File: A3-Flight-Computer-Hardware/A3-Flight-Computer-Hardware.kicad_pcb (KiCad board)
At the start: 2 copper layers, 50 x 50 mm, 57 parts, among them J1 BAT, J2 ST1W008S4ER1500, J3 USB_C_Receptacle_USB2.0_14P, J4 Cam 1, J5 Debug Header, J6 Cam 2, J7 Cam 3, J8 Telem, J9 CAN, SW1 BOOT, SW2 RST, U1 STM32H523RETx, U2 ADXL375BCCZ-RL7, U3 LSM6DSO32TR, U4 LPS22HBTR, U5 PTCAN3414DR, Y1 TSX-3225_16.0000MF18X-AC0, Y2 ECS-.327-9-34QCS-TR

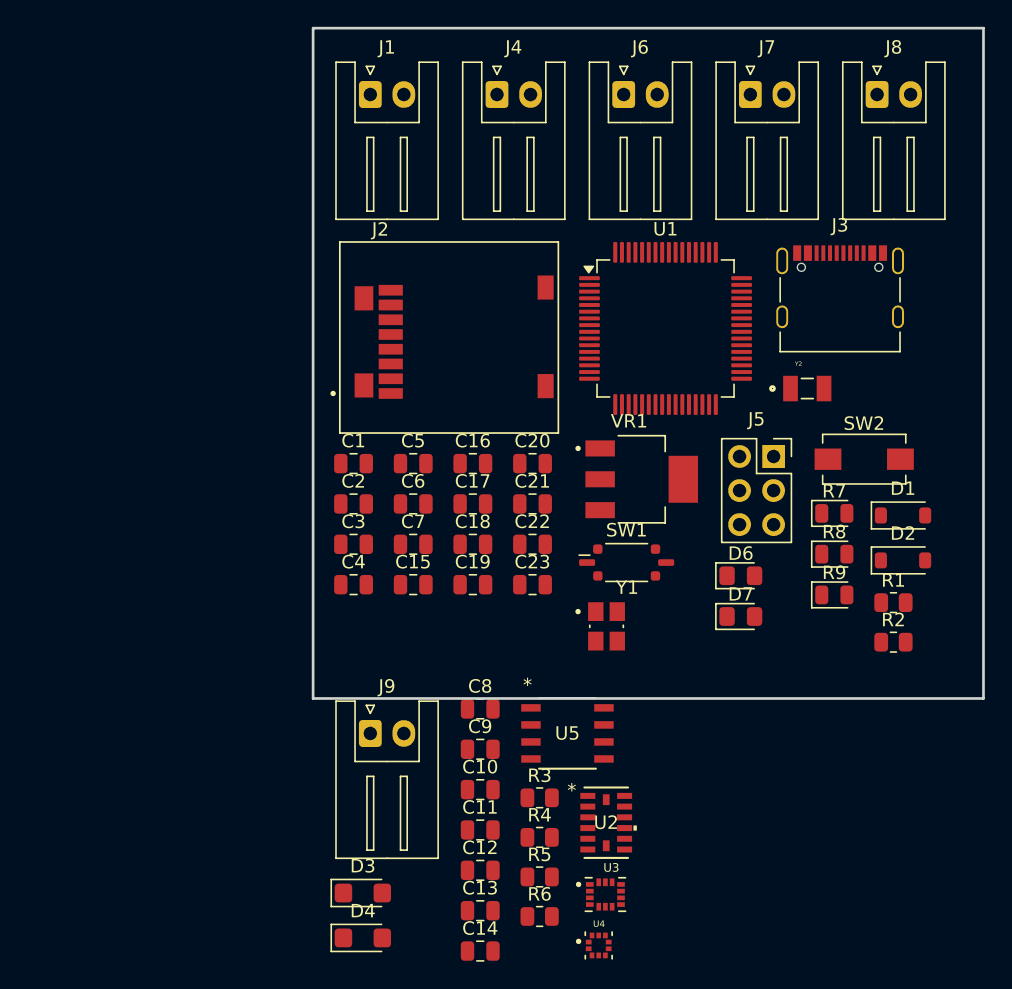
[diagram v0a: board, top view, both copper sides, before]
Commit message: First PCB revision
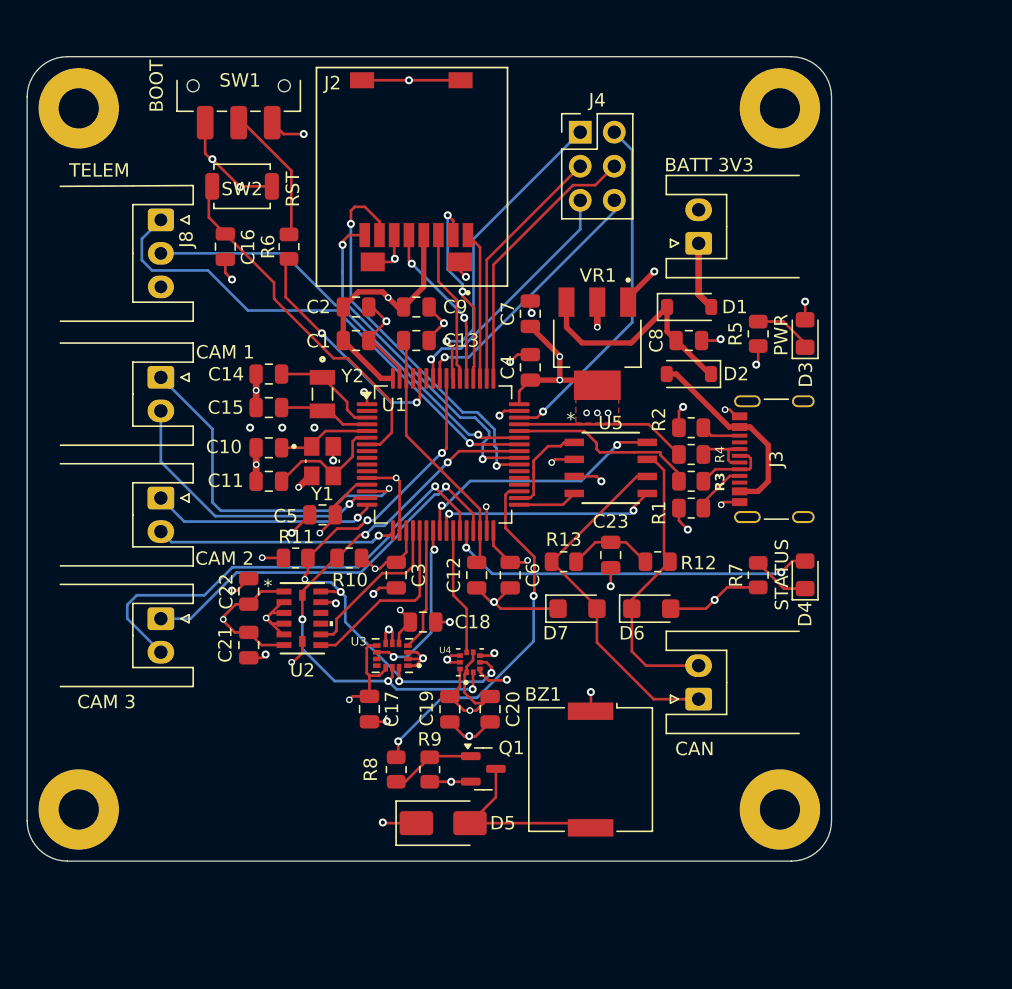
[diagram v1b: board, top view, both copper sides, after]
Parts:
- added BZ1: Buzzer, Buzzer_Beeper:Buzzer_Murata_PKMCS0909E, F.Cu at (159.5, 131.0)
- added D5: SS14, Diode_SMD:D_SMA, F.Cu at (148.5, 135.0)
- added Q1: IRLML0030, Package_TO_SOT_SMD:SOT-23, F.Cu at (151.5, 130.9)
- added R10: 1.8k, Resistor_SMD:R_0805_2012Metric, F.Cu at (141.5, 115.2)
- added R11: 1.8k, Resistor_SMD:R_0805_2012Metric, F.Cu at (137.5, 115.2)
- added R12: 60, Resistor_SMD:R_0805_2012Metric, F.Cu at (164.5, 115.5)
- added R13: 60, Resistor_SMD:R_0805_2012Metric, F.Cu at (157.5, 115.5)
- added REF**: MountingHole_3mm_Pad, MountingHole:MountingHole_3mm_Pad, F.Cu at (173.6, 134.0)
- added REF**: MountingHole_3mm_Pad, MountingHole:MountingHole_3mm_Pad, F.Cu at (173.6, 81.7)
- added REF**: MountingHole_3mm_Pad, MountingHole:MountingHole_3mm_Pad, F.Cu at (121.3, 81.7)
- added REF**: MountingHole_3mm_Pad, MountingHole:MountingHole_3mm_Pad, F.Cu at (121.3, 134.0)
- C1: value 22uF -> 4.7uF
- C10, C11: value 100nF -> 8pF
- C12, C13: value 100nF -> 2.2uF
- C14: value 4.7nF -> 16pF
- C15: value 2.2uF -> 16pf
- C16: value 2.2uF -> 100nF
- C2: value 10uF -> 100nF
- C22: value 4.7uF -> 100nF
- C23: value 100nF -> 4.7nF
- C4, C5: value 8pF -> 100nF
- C6: value 4pF -> 100nF
- C7: value 4pF -> 22uF
- C8: value 100nF -> 10uF
- D3, D4: value SMF54CA -> LED; footprint Diode_SMD:D_SMF -> LED_SMD:LED_0805_2012Metric_Pad1.15x1.40mm_HandSolder
- D6, D7: value LED -> SMF54CA; footprint LED_SMD:LED_0805_2012Metric_Pad1.15x1.40mm_HandSolder -> Diode_SMD:D_SMF
- J4: value Cam 1 -> Debug Header; footprint Connector_JST:JST_XH_S2B-XH-A_1x02_P2.50mm_Horizontal -> Connector_PinHeader_2.54mm:PinHeader_2x03_P2.54mm_Vertical
- J5: value Debug Header -> Cam 1; footprint Connector_PinSocket_2.54mm:PinSocket_2x03_P2.54mm_Vertical -> Connector_JST:JST_XH_S2B-XH-A_1x02_P2.50mm_Horizontal
- J8: footprint Connector_JST:JST_XH_S2B-XH-A_1x02_P2.50mm_Horizontal -> Connector_JST:JST_XH_S3B-XH-A_1x03_P2.50mm_Horizontal
- R3, R4: value 1.8k -> 27R
- R5: value 60 -> 240R
- R6: value 60 -> 10k
- R7: value 10k -> 240R; footprint LED_SMD:LED_0805_2012Metric -> Resistor_SMD:R_0805_2012Metric
- R8: value 240R -> 100; footprint LED_SMD:LED_0805_2012Metric -> Resistor_SMD:R_0805_2012Metric
- R9: value 240R -> 100k; footprint LED_SMD:LED_0805_2012Metric -> Resistor_SMD:R_0805_2012Metric
- SW1: footprint Button_Switch_SMD:SW_DIP_SPSTx01_Slide_Copal_CVS-01xB_W5.9mm_P1mm -> Button_Switch_SMD:SW_SPDT_CK_JS102011SAQN
- SW2: footprint Button_Switch_SMD:SW_SPST_EVQPE1 -> Button_Switch_SMD:SW_SPST_TS-1088-xR025
- moved J7 59.3 mm to (127.2, 120.2), turned to -90 degrees
- moved J8 54.2 mm to (127.4, 90.0), turned to -90 degrees
- moved R6 53.3 mm to (137.0, 92.0), turned to -90 degrees
- moved D3 53.2 mm to (175.5, 98.5), turned to 90 degrees
- moved SW2 50.7 mm to (133.5, 87.5), turned to 180 degrees
- moved J5 46.1 mm to (127.4, 101.8), turned to -90 degrees
- moved J6 45.9 mm to (127.2, 110.7), turned to -90 degrees
- moved SW1 45.8 mm to (133.2, 80.0), turned to 180 degrees
- moved C14 45.8 mm to (135.5, 101.5), turned to 180 degrees
- moved R5 43.7 mm to (172.0, 98.5), turned to 90 degrees
- moved C13 42.8 mm to (146.5, 99.0)
- moved D4 42.7 mm to (175.5, 116.5), turned to 90 degrees
- moved R8 36.4 mm to (145.0, 131.0), turned to -90 degrees
- moved Y2 36.2 mm to (139.5, 103.0), turned to -90 degrees
- moved C9 33.3 mm to (146.5, 96.5)
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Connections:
- C10 pad 1: +3.3V -> /HSE_IN
- C11 pad 1: +3.3V -> /HSE_OUT
- C12 pad 1: +3.3V -> Net-(C12-Pad1)
- C13 pad 1: +3.3V -> Net-(C12-Pad1)
- C14 pad 1: Net-(C14-Pad1) -> /LSE_IN
- C15 pad 1: Net-(C15-Pad1) -> /LSE_OUT
- C16 pad 1: Net-(C15-Pad1) -> /RST
- C2 pad 1: Net-(D1-K) -> +3.3V
- C23 pad 1: /RST -> Net-(C23-Pad1)
- C4 pad 1: /HSE_IN -> +3.3V
- C5 pad 1: /HSE_OUT -> +3.3V
- C6 pad 1: /LSE_IN -> +3.3V
- C7 pad 1: /LSE_OUT -> +3.3V
- C8 pad 1: +3.3V -> Net-(D1-K)
- D3 pad 1: Net-(D3-A1) -> Net-(D3-K)
- D3 pad 2: GND -> +3.3V
- D4 pad 1: GND -> Net-(D4-K)
- D4 pad 2: Net-(D4-A2) -> /STAT_LED
- D6 pad 1: Net-(D6-K) -> Net-(D6-A1)
- D6 pad 2: +3.3V -> GND
- D7 pad 1: Net-(D7-K) -> GND
- D7 pad 2: /STAT_LED -> Net-(D7-A2)
- J3 pad A6: /USB_DP -> Net-(J3-D+-PadA6)
- J3 pad A7: /USB_DM -> Net-(J3-D--PadA7)
- J3 pad B6: /USB_DP -> Net-(J3-D+-PadA6)
- J3 pad B7: /USB_DM -> Net-(J3-D--PadA7)
- J4 pad 1: /CAM1_TX -> /JTDO-SWO
- J4 pad 2: /CAM1_RX -> /JTMS-SWDIO
- J5 pad 1: /JTMS-SWDIO -> /CAM1_TX
- J5 pad 2: /JTDO-SWO -> /CAM1_RX
- J9 pad 1: Net-(D4-A2) -> Net-(D7-A2)
- J9 pad 2: Net-(D3-A1) -> Net-(D6-A1)
- R3 pad 1: +3.3V -> /USB_DM
- R3 pad 2: /I2C_SCL -> Net-(J3-D--PadA7)
- R4 pad 1: +3.3V -> /USB_DP
- R4 pad 2: /I2C_SDA -> Net-(J3-D+-PadA6)
- R5 pad 1: Net-(C14-Pad1) -> GND
- R5 pad 2: Net-(D3-A1) -> Net-(D3-K)
- R6 pad 1: Net-(D4-A2) -> Net-(SW1-B)
- R6 pad 2: Net-(C14-Pad1) -> /BOOT
- R7 pad 1: Net-(SW1-B) -> GND
- R7 pad 2: /BOOT -> Net-(D4-K)
- R8 pad 1: GND -> /BUZZ
- R8 pad 2: Net-(D6-K) -> Net-(Q1-G)
- R9 pad 2: Net-(D7-K) -> Net-(Q1-G)
- U1 pad 20: /ADXL375_INT1 -> /ADXL375_INT2
- U1 pad 21: /ADXL375_INT2 -> /ADXL375_INT1
- U1 pad 30: Net-(C15-Pad1) -> Net-(C12-Pad1)
- U1 pad 35: unconnected-(U1-PB14-Pad35) -> /BUZZ
- U1 pad 62: Net-(C15-Pad1) -> Net-(C12-Pad1)
- U5 pad 6: Net-(D4-A2) -> Net-(D7-A2)
- U5 pad 7: Net-(D3-A1) -> Net-(D6-A1)
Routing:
- net GND: track 0.00 -> 119.5 mm, vias 0 -> 46
- net +3.3V: track 0.00 -> 96.8 mm, vias 0 -> 22
- net /I2C_SDA: track 0.00 -> 43.3 mm, vias 0 -> 6
- net /I2C_SCL: track 0.00 -> 41.2 mm, vias 0 -> 5
- net /TELEM_TX: track 0.00 -> 37.4 mm, vias 0 -> 1
- net /CAM3_RX: track 0.00 -> 35.4 mm, vias 0 -> 1
- net /TELEM_RX: track 0.00 -> 32.4 mm, vias 0 -> 1
- net /CAM3_TX: track 0.00 -> 29.8 mm, vias 0 -> 1
- net /SD_D0: track 0.00 -> 29.6 mm, vias 0 -> 2
- net /STAT_LED: track 0.00 -> 27.8 mm, vias 0 -> 2
- net /BUZZ: track 0.00 -> 27.4 mm, vias 0 -> 2
- net /CAM1_TX: track 0.00 -> 26.8 mm, vias 0 -> 1
- net Net-(D7-A2): track 0.00 -> 26.5 mm
- net /RST: track 0.00 -> 26.4 mm
- net /SD_D1: track 0.00 -> 26.2 mm, vias 0 -> 2
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- added copper zone on F.Cu, net +3.3V
- added copper zone on In2.Cu, net +3.3V
- added copper zone on In1.Cu, net GND
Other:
- board size 50 x 50 mm -> 60 x 60 mm
- copper layers 2 -> 4
- board text added: "BATT 3V3"
- board text added: "BOOT"
- board text added: "CAM 1"
- board text added: "CAM 2"
- board text added: "CAM 3"
- board text added: "CAN"
- board text added: "PWR"
- board text added: "RST"
- board text added: "STATUS"
- board text added: "TELEM"
